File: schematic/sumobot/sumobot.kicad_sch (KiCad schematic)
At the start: 10 parts, among them J1 Screw_Terminal_01x02, J2 Screw_Terminal_01x02, J3 Screw_Terminal_01x02, J4 Conn_01x05, J5 Screw_Terminal_01x02, J6 Screw_Terminal_01x02, J7 Conn_01x05, U1 ROB-14450, U2 ROB-14450

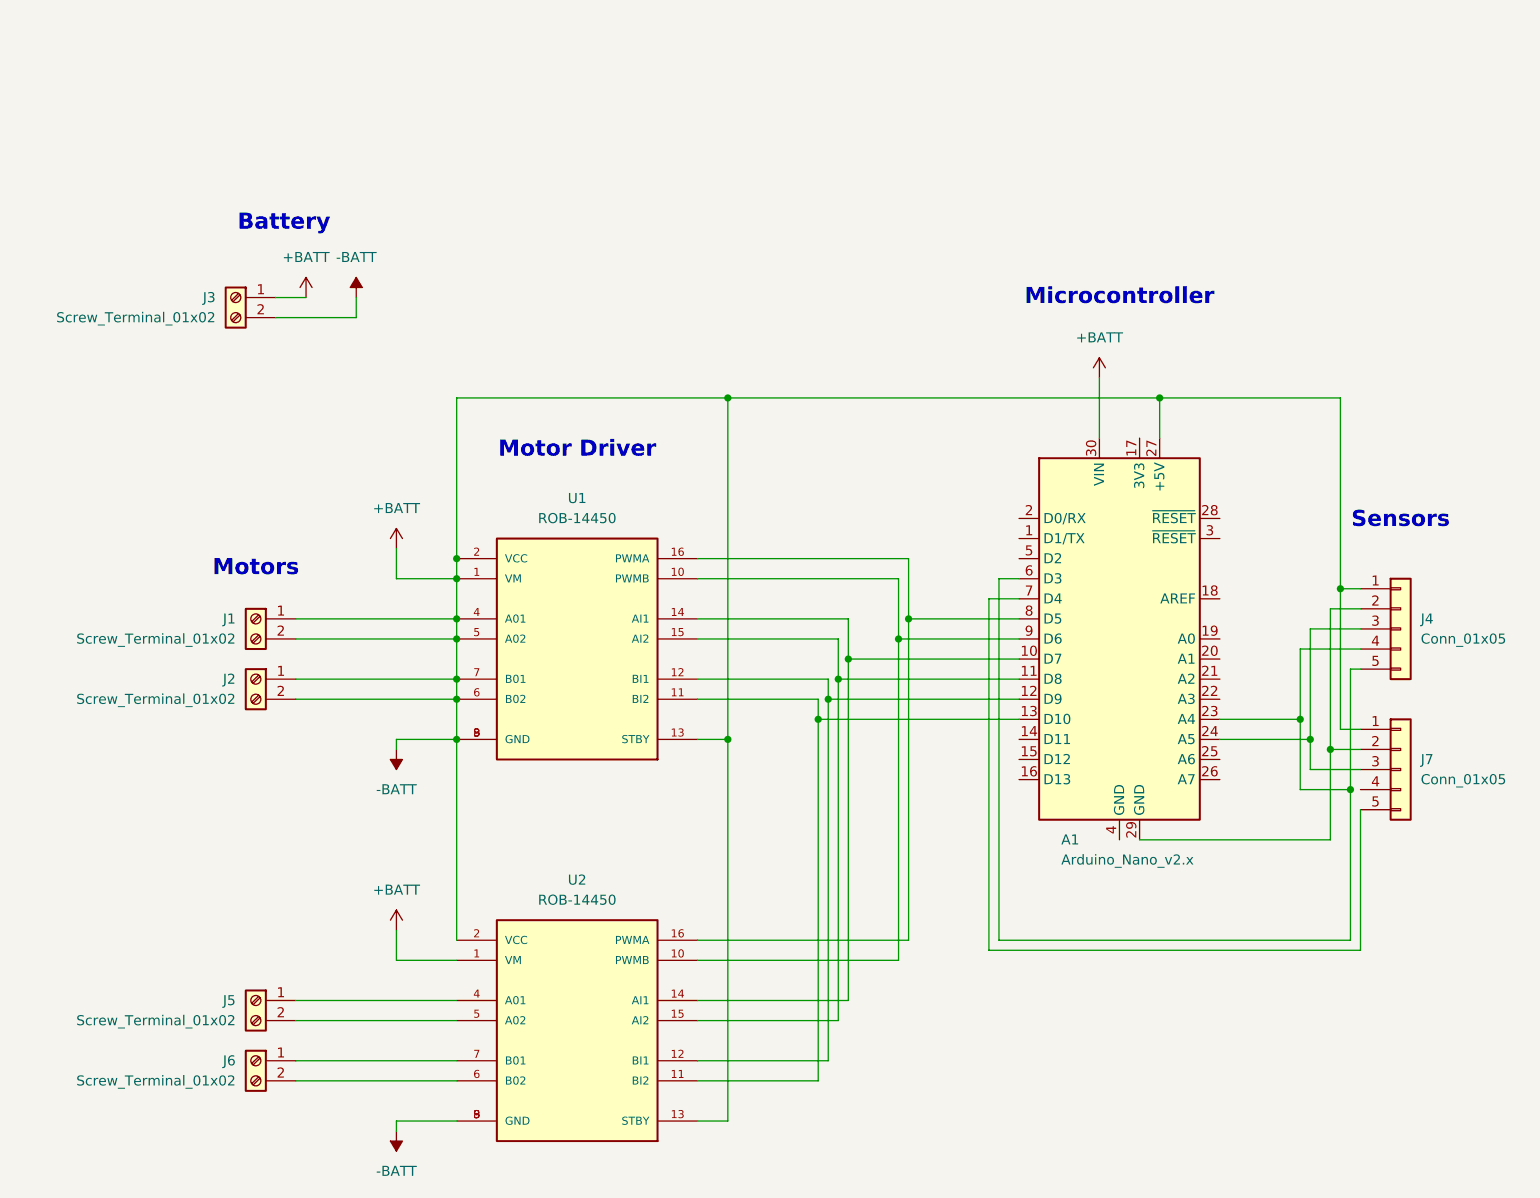
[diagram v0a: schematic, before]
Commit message: haha
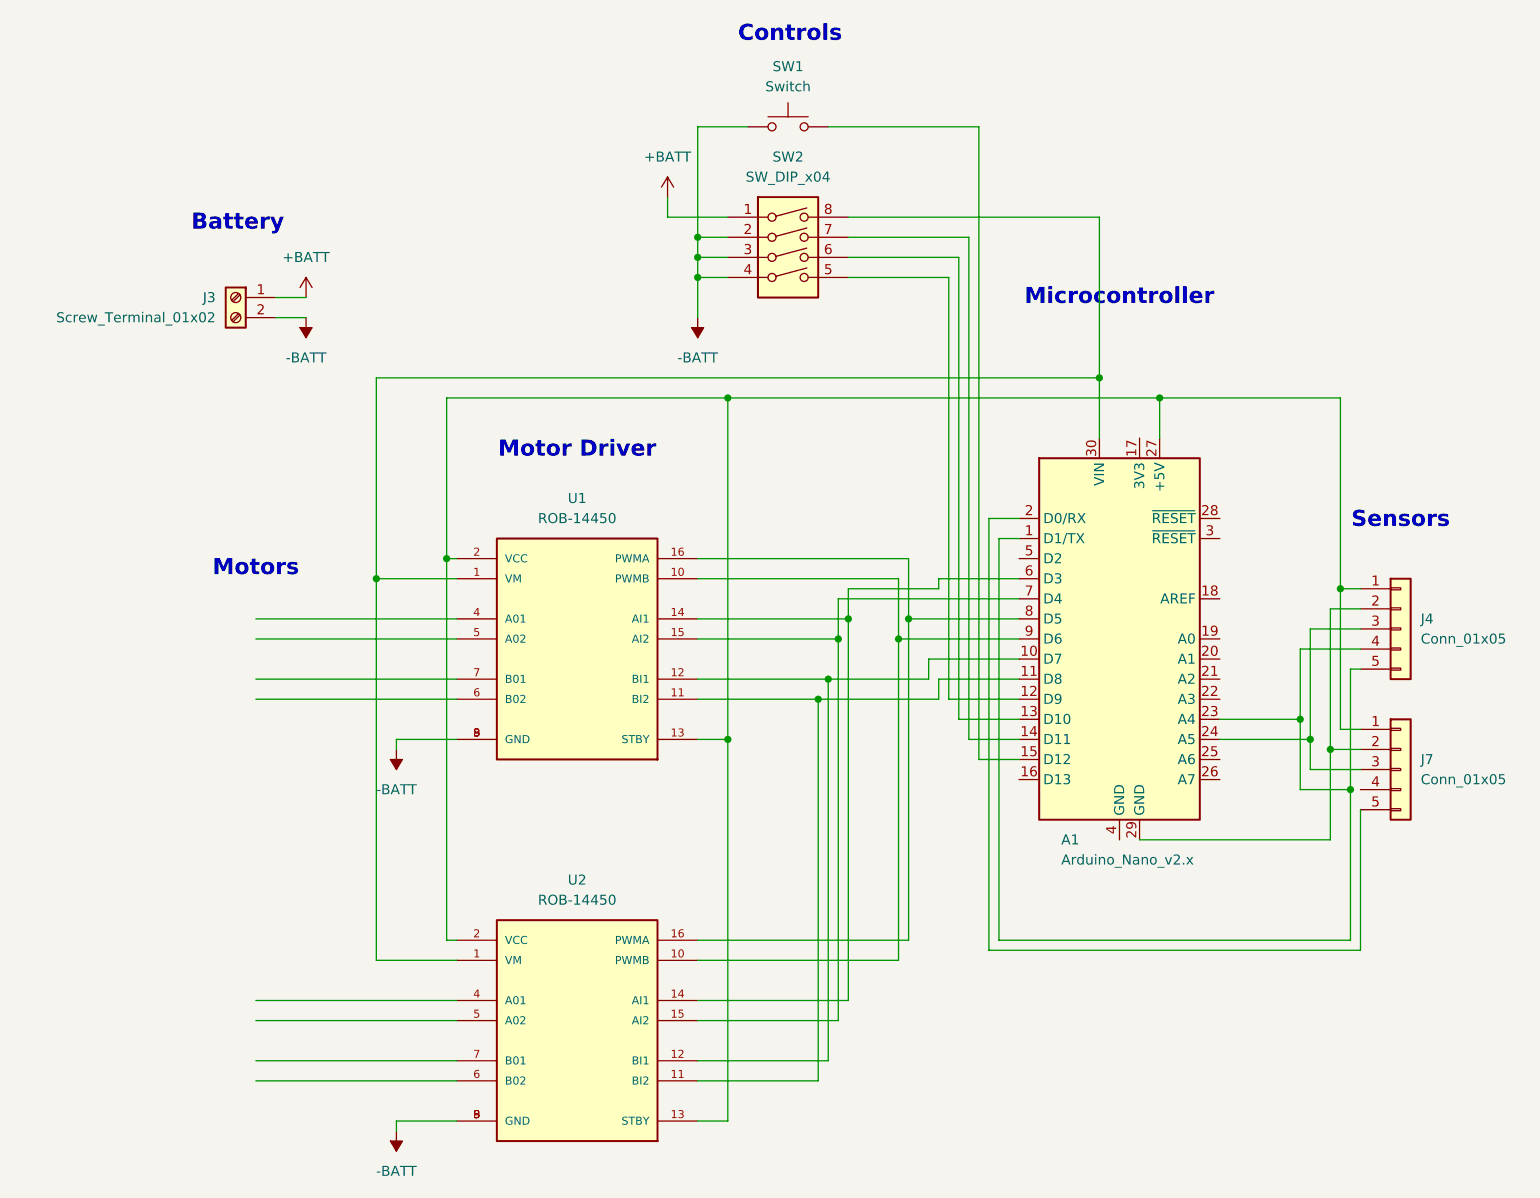
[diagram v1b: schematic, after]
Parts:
- removed J1, J2, J5, J6: Screw_Terminal_01x02, TerminalBlock:TerminalBlock_MaiXu_MX126-5.0-02P_1x02_P5.00mm, symbol Connector:Screw_Terminal_01x02
- added SW1: Switch, symbol ScottoKeebs:Placeholder_Switch
- added SW2: SW_DIP_x04, symbol Switch:SW_DIP_x04
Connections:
- net +BATT: now also SW2.1; no longer A1.27 (+5V), A1.30 (VIN), J3.2 (Pin_2), J4.1 (Pin_1), J7.1 (Pin_1), U1.1 (VM), U1.13 (STBY), U1.2 (VCC), U1.3 (GND), U1.4 (A01), U1.5 (A02), U1.6 (B02), U1.7 (B01), U1.8 (GND), U1.9 (GND), U2.1 (VM), U2.13 (STBY), U2.2 (VCC), U2.3 (GND), U2.8 (GND), U2.9 (GND)
- net at U1.11 (BI2), U2.11 (BI2): now also A1.11 (D8); no longer A1.13 (D10)
- net at U1.12 (BI1), U2.12 (BI1): now also A1.10 (D7); no longer A1.12 (D9)
- net at U1.14 (AI1), U2.14 (AI1): now also A1.6 (D3); no longer A1.10 (D7)
- net at U1.15 (AI2), U2.15 (AI2): now also A1.7 (D4); no longer A1.11 (D8)
- net at A1.23 (A4), J4.4 (Pin_4), J4.5 (Pin_5): now also A1.1 (D1/TX); no longer A1.6 (D3)
- net at A1.14 (D11): now also SW2.7
- net at A1.15 (D12): now also SW1.2
- net at A1.2 (D0/RX): now also J7.5 (Pin_5)
- new net: A1.30 (VIN), SW2.8, U1.1 (VM), U2.1 (VM)
- new net: A1.27 (+5V), J4.1 (Pin_1), J7.1 (Pin_1), U1.13 (STBY), U1.2 (VCC), U2.13 (STBY), U2.2 (VCC)
- new net: A1.12 (D9), SW2.5
- new net: A1.13 (D10), SW2.6
- new net -BATT: J3.2 (Pin_2), SW1.1, SW2.2, SW2.3, SW2.4, U1.3 (GND), U1.8 (GND), U1.9 (GND), U2.3 (GND), U2.8 (GND), U2.9 (GND)
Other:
- note added: "Controls"
